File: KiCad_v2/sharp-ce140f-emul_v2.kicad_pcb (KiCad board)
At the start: 2 copper layers, 58.6 x 36 mm, 50 parts, among them J1 ext pins, J2 Sharp PC 11-pin, J3 USB_B_Micro, J4 Micro_SD_Card_Det, J5 Battery, J6 SWD, SW1 AYZ0102AGRLC, U1 TXS0108EPW, U2 STM32L432KCUx, U4 MCP73831, U5 XC6206P332MR, Y1 32.768KHz

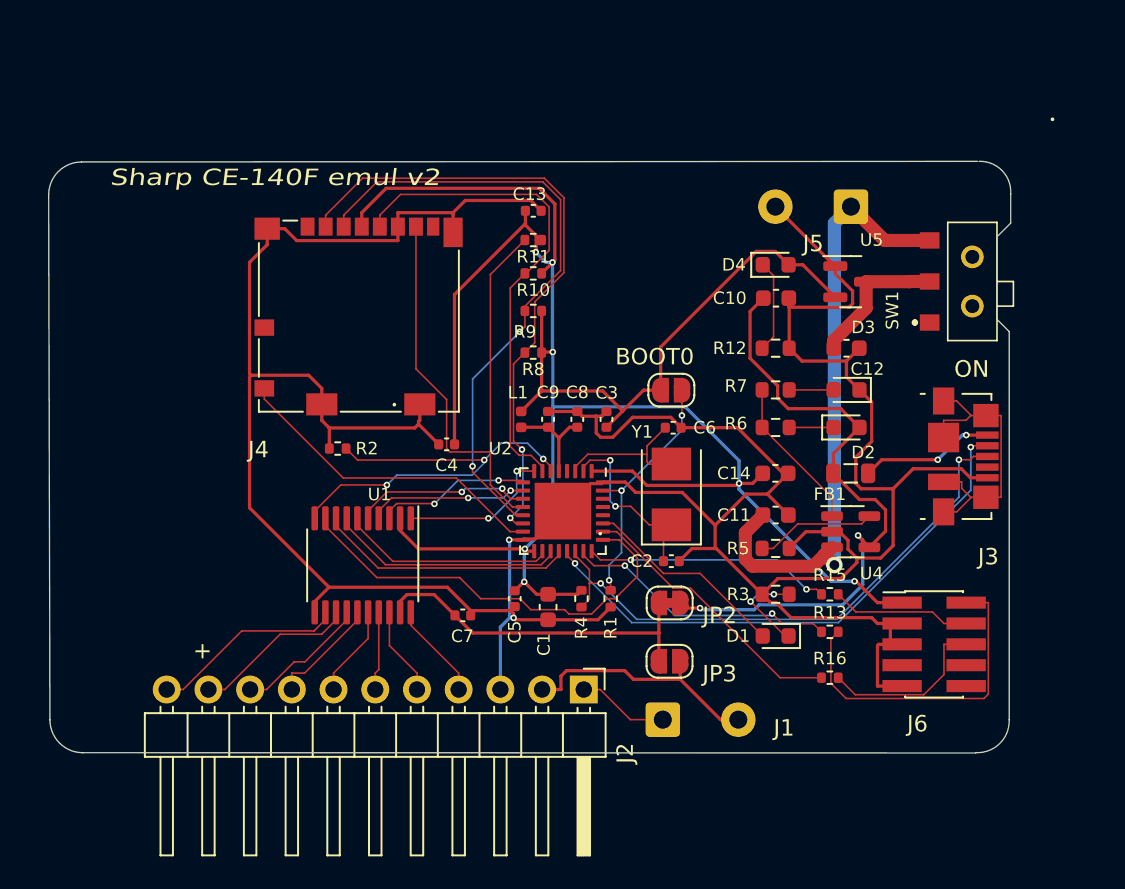
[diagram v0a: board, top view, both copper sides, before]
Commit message: DRAFT v2 schematics revisions
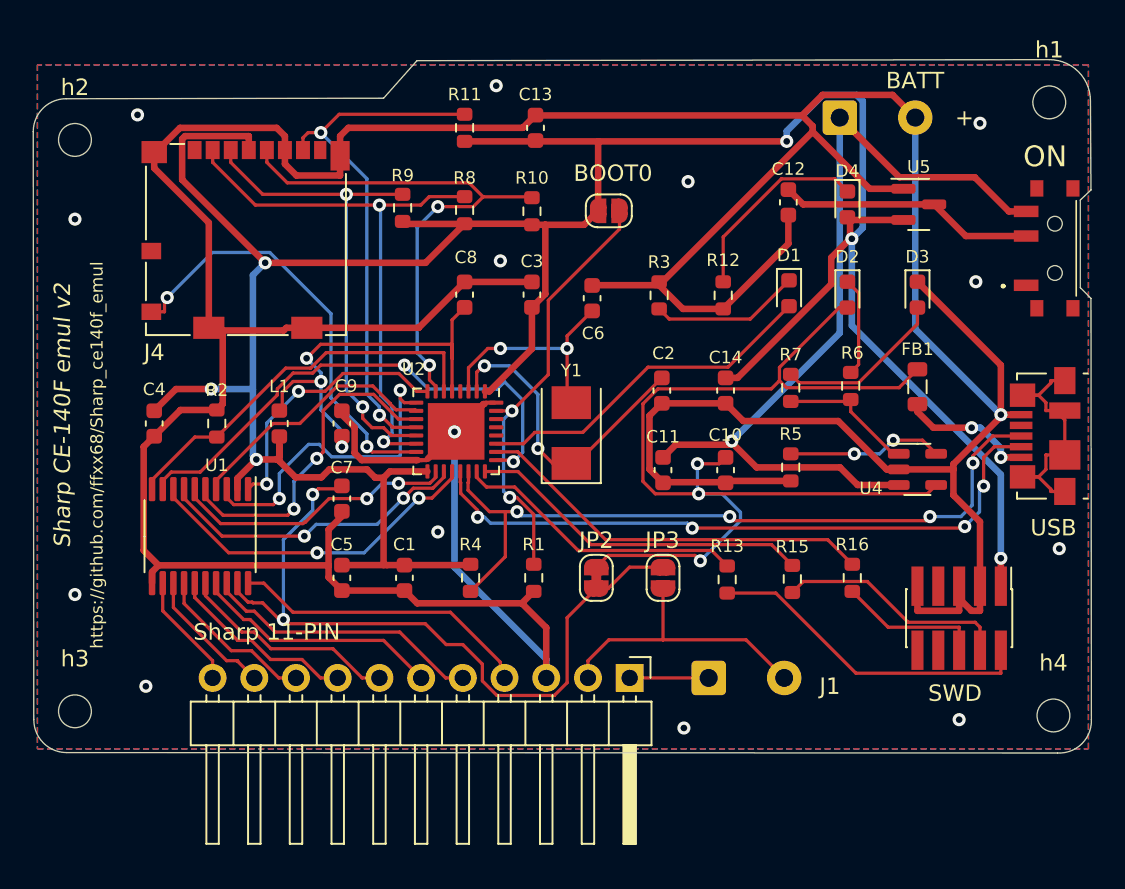
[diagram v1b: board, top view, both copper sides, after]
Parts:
- removed J3: USB_B_Micro, Connector_USB:USB_Micro-B_Molex_47346-0001
- removed J5: Battery, Connector_Wire:SolderWire-0.5sqmm_1x02_P4.6mm_D0.9mm_OD2.1mm
- removed J6: SWD, Connector_PinHeader_1.27mm:PinHeader_2x05_P1.27mm_Vertical_SMD
- removed JP1: BOOT0, Jumper:SolderJumper-2_P1.3mm_Open_RoundedPad1.0x1.5mm
- removed SW1: AYZ0102AGRLC, SamacSys_Parts:AYZ0102AGRLC
- added BATT: Battery, Connector_Wire:SolderWire-0.5sqmm_1x02_P4.6mm_D0.9mm_OD2.1mm, F.Cu at (174.3, 83.7)
- added BOOT0: BOOT0, Jumper:SolderJumper-2_P1.3mm_Open_RoundedPad1.0x1.5mm, F.Cu at (160.3, 89.4)
- added ON: PCM12SMTR, ce140f_library:PCM12SMTR, F.Cu at (187.4, 91.7)
- added SWD: SWD, Connector_PinHeader_1.27mm:PinHeader_2x05_P1.27mm_Vertical_SMD, F.Cu at (181.6, 114.2)
- added USB: USB_B_Micro, Connector_USB:USB_Micro-B_Molex_47346-0001, F.Cu at (186.8, 103.1)
- added h1: MountingHole_2mm, MountingHole:MountingHole_2mm, F.Cu at (187.1, 82.8)
- added h2: MountingHole_2mm, MountingHole:MountingHole_2mm, F.Cu at (127.8, 85.1)
- added h3: MountingHole_2mm, MountingHole:MountingHole_2mm, F.Cu at (127.8, 119.9)
- added h4: MountingHole_2mm, MountingHole:MountingHole_2mm, F.Cu at (187.4, 120.1)
- C1, C10, C11, C12, C14: footprint Capacitor_SMD:C_0603_1608Metric -> ce140f_library:C_0603_1608Metric
- C13, C2, C3, C4, C5, C6, C7, C8, C9: footprint Capacitor_SMD:C_0402_1005Metric -> ce140f_library:C_0603_1608Metric
- L1: footprint Inductor_SMD:L_0402_1005Metric -> Inductor_SMD:L_0603_1608Metric
- R1, R10, R11, R13, R15, R16, R2, R4, R8, R9: footprint Resistor_SMD:R_0402_1005Metric -> ce140f_library:R_0603_1608Metric
- R12, R3, R5, R6, R7: footprint Resistor_SMD:R_0603_1608Metric -> ce140f_library:R_0603_1608Metric
- Sharp 11-PIN: renamed from J2
- moved D1 20.9 mm to (171.2, 94.4), turned to -90 degrees
- moved R3 19.5 mm to (163.3, 94.6), turned to 90 degrees
- moved C4 17.9 mm to (132.6, 102.4), turned to -90 degrees
- moved L1 14.7 mm to (140.2, 102.4), turned to 90 degrees
- moved C9 12.6 mm to (144.0, 102.4)
- moved C10 10.9 mm to (167.4, 105.2), turned to -90 degrees
- moved C5 10.6 mm to (144.0, 111.8)
- moved C2 10.4 mm to (163.5, 100.4), turned to -90 degrees
- moved C7 10.2 mm to (144.0, 106.9), turned to -90 degrees
- moved C8 10.2 mm to (151.5, 94.5)
- moved R9 10.1 mm to (147.7, 89.2), turned to 90 degrees
- moved U1 10.1 mm to (135.4, 109.2)
- moved R8 9.63 mm to (151.5, 89.4), turned to 90 degrees
- moved C12 9.56 mm to (171.2, 88.9), turned to -90 degrees
- moved C6 9.31 mm to (159.3, 94.7), turned to 90 degrees
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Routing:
- net GND: track 213.0 -> 292.5 mm, vias 2 -> 15
- net +3V3: track 144.2 -> 180.5 mm, vias 7 -> 6
- net VPP: track 39.1 -> 65.0 mm, vias 2 -> 3
- net /vccb: track 21.1 -> 45.3 mm, vias 0 -> 2
- net +3.3VA: track 5.97 -> 26.3 mm, vias 0 -> 3
- net unconnected-(J3-Pad6): track 17.8 -> 0.00 mm
- net /V_BAT: track 37.8 -> 52.1 mm
- net unconnected-(J3-Shield-Pad6): track 0.00 -> 13.9 mm
- net /busy: track 5.91 -> 18.4 mm
- net /dout: track 5.40 -> 17.1 mm
- net /BOOT0: track 15.2 -> 26.4 mm, vias 3 -> 2
- net USB_D+: track 34.5 -> 45.2 mm, vias 2 -> 4
- net /x_in: track 4.79 -> 15.2 mm
- net PA3: track 9.42 -> 19.6 mm
- net PA5: track 10.8 -> 19.9 mm
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- added copper zone on B.Cu, net GND
- added copper zone on F.Cu, net GND
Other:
- board size 58.6 x 36 mm -> 64.4 x 42.2 mm
- board text added: "https://github.com/ffxx68/Sharp_ce140f_emul"
- board text removed: "ON"
